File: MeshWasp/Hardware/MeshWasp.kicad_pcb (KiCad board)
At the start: 2 copper layers, 25.8 x 28.1 mm, 14 parts, among them SW1 RST, U1 CONN_MICROSD, U2 XBEE

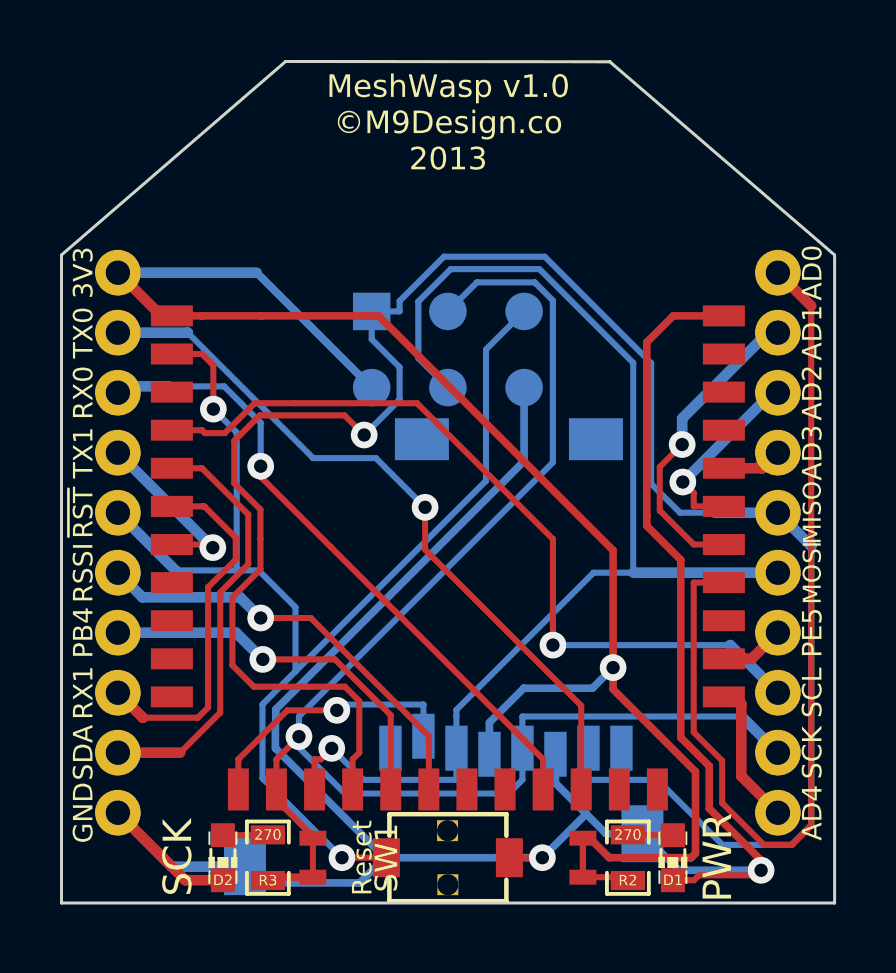
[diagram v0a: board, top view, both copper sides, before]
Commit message: Minor silks & logo work.
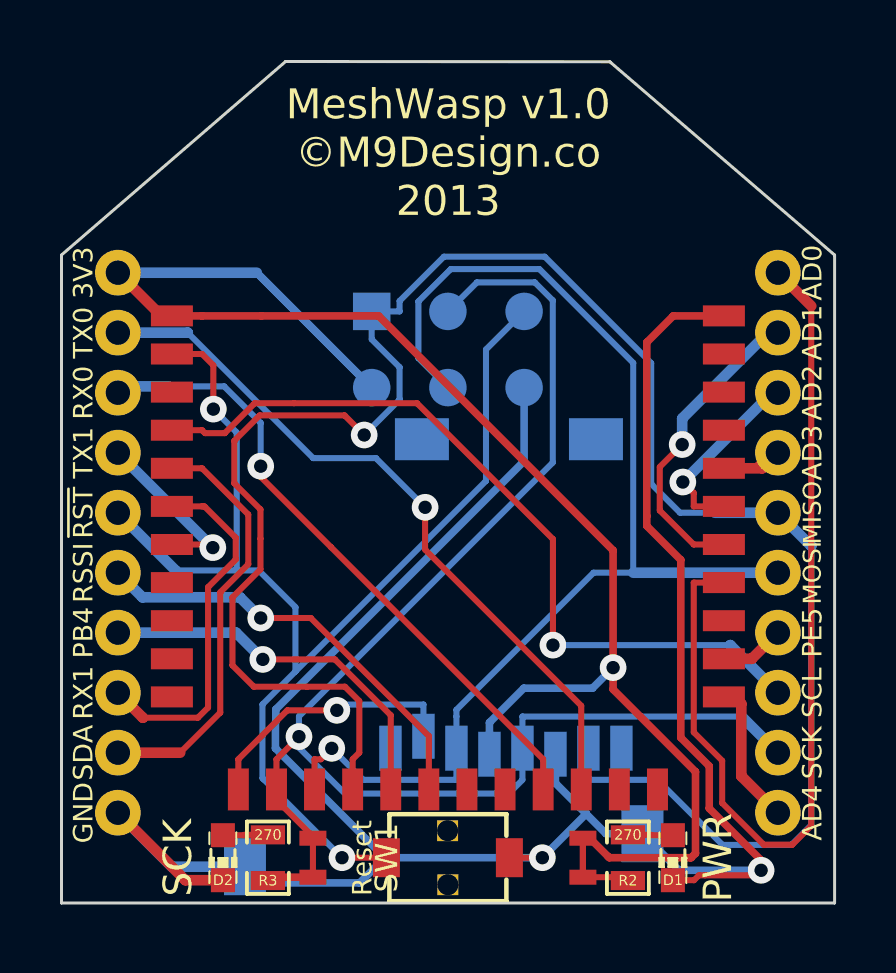
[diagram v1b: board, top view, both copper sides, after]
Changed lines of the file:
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@@
     (links 44)
     (no_connects 0)
-    (area 137.069999 92.909999 162.940001 121.060001)
+    (area 135.5699 92.646799 162.940001 121.228201)
     (thickness 1.6)
     (drawings 13)
@@
     (18 B.Paste user)
     (19 F.Paste user)
-    (20 B.SilkS user hide)
+    (20 B.SilkS user)
     (21 F.SilkS user)
-    (22 B.Mask user hide)
-    (23 F.Mask user hide)
+    (22 B.Mask user)
+    (23 F.Mask user)
     (24 Dwgs.User user)
     (25 Cmts.User user)
-    (26 Eco1.User user)
+    (26 Eco1.User user hide)
     (27 Eco2.User user)
     (28 Edge.Cuts user)
@@
     (effects (font (size 0.75 0.75) (thickness 0.1875)) (justify mirror))
   )
-  (gr_text "MeshWasp v1.0\n©M9Design.co \n2013" (at 150.01 95) (layer F.SilkS)
-    (effects (font (size 0.75 0.75) (thickness 0.1875)))
+  (gr_text "MeshWasp v1.0\n©M9Design.co \n2013" (at 150.01 96) (layer F.SilkS)
+    (effects (font (size 1 1) (thickness 0.1875)))
   )
   (gr_text "by\nRobert\nPowers" (at 156 103) (layer B.SilkS)
